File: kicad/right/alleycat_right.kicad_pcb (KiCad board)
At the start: 2 copper layers, 134 x 128 mm, 116 parts, among them J1 Conn_01x04_Male, J2 USB_C_Receptacle_USB2.0, SW1 SW_Push, U1 nRF52840_holyiot_18010, U2 TP4056, U3 DW01A, U4 FS8205, U5 SRV05-4, U6 XC6206PxxxMR

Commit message: swag
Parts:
- U1: footprint E73-2G4M08S1C:E73-2G4M08S1C -> marbastlib-various:nRF52840_holyiot_18010
- moved U5 83.2 mm to (19.0, 102.0)
- moved J2 76.2 mm to (-22.0, 20.6)
- moved D40 65.0 mm to (18.0, 117.0)
- moved D41 65.0 mm to (32.0, 117.0)
- moved D42 65.0 mm to (18.0, 103.0)
- moved D46 65.0 mm to (22.0, 109.0)
- moved Dr 65.0 mm to (32.0, 103.0)
- moved S1 65.0 mm to (25.0, 110.0)
- moved U6 64.8 mm to (1.00, 89.0)
- moved U4 62.9 mm to (3.00, 100.0)
- moved F1 42.2 mm to (-2.00, 75.0)
- moved SW1 39.0 mm to (-11.0, 127.0)
- moved D44 23.9 mm to (7.00, 97.0)
- moved U2 8.06 mm to (31.0, 102.0)
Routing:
- added copper zone on B.Cu, net GND

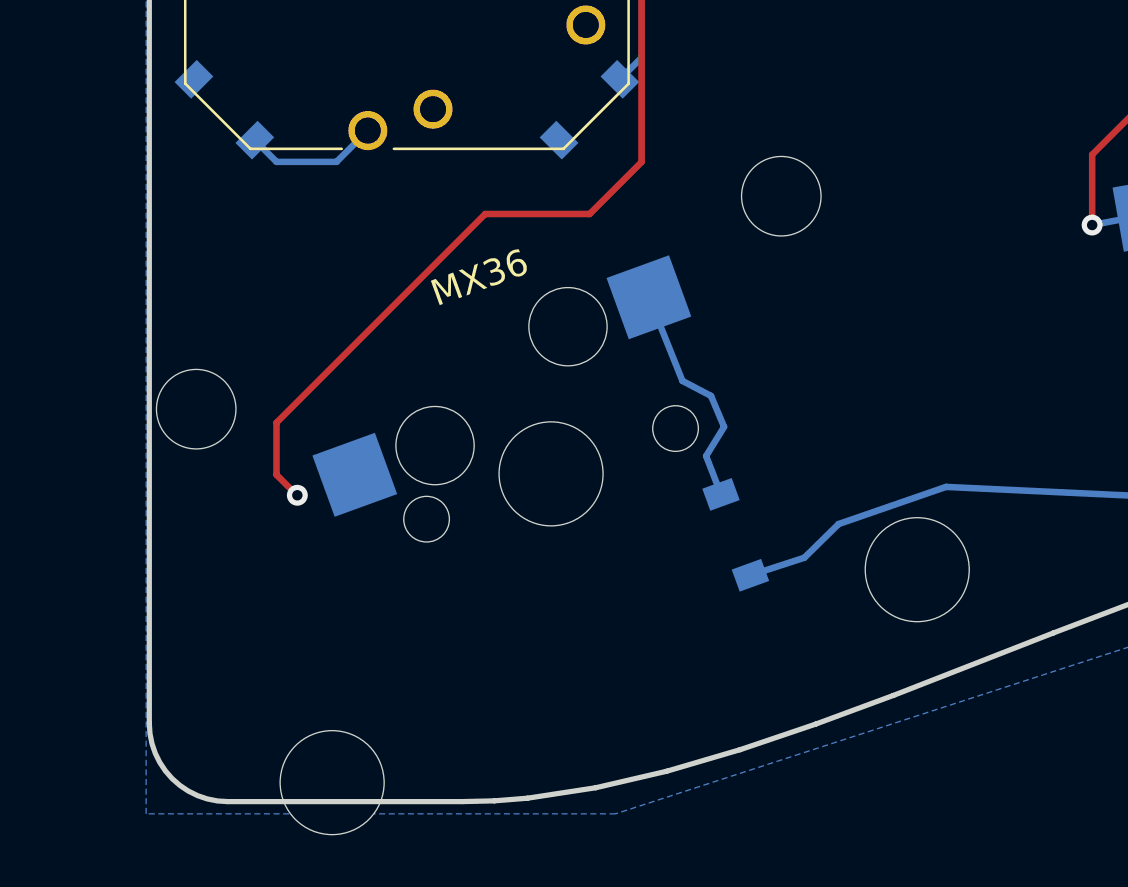
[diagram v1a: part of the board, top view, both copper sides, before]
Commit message: nya
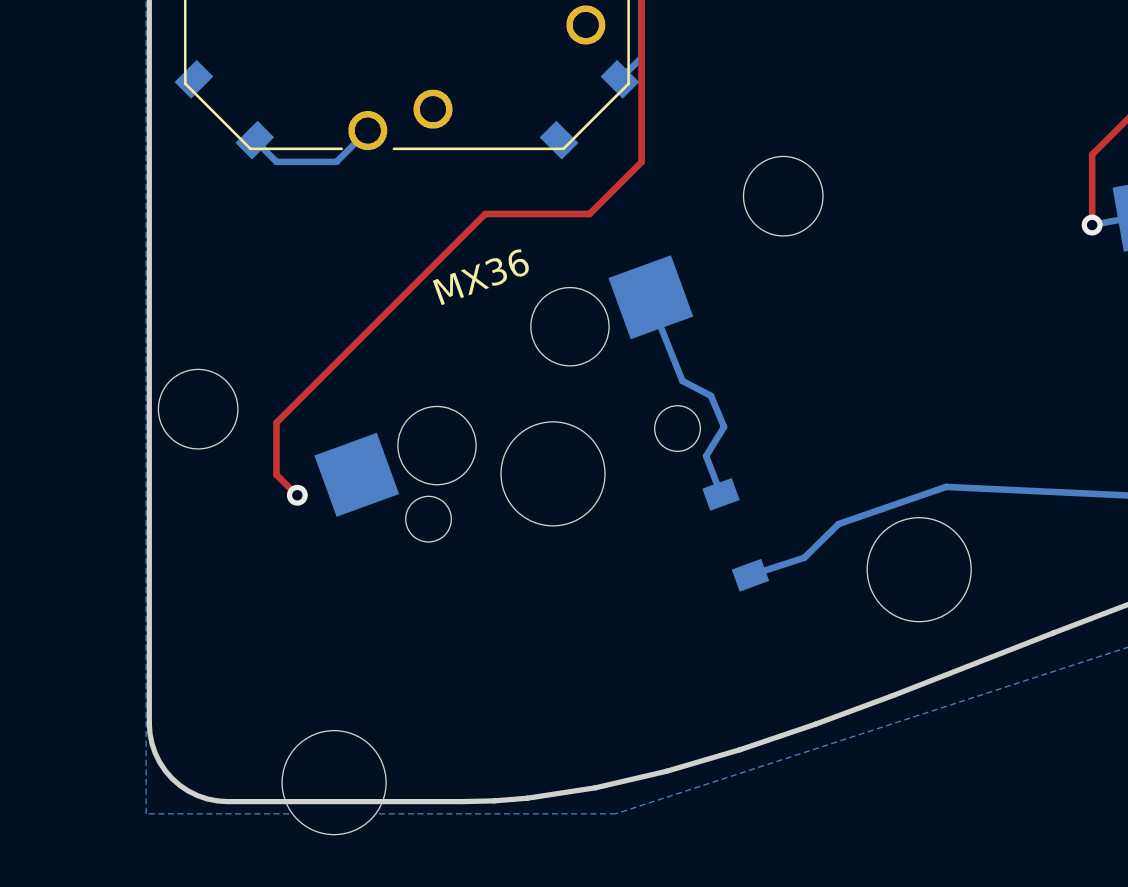
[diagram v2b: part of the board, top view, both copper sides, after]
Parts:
- moved MX36 0.07 mm to (23.1, 131.0)
